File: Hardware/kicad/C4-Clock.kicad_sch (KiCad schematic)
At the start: 39 parts, among them J1 Keypad, J2 Battery, J3 LCD1602, J4 Boost Module, J5 ICSP, K1 FINDER-36.11-5V, Q1 S9014, Q2 S9014, Q3 S9014, SW1 SW_SPST, SW2 SW_SPST, U1 ATmega328P-P, U2 AMS1117-5.0, U3 PCF8574A, U4 DS1302+, Y1 16MHz, Y2 32.768kHz

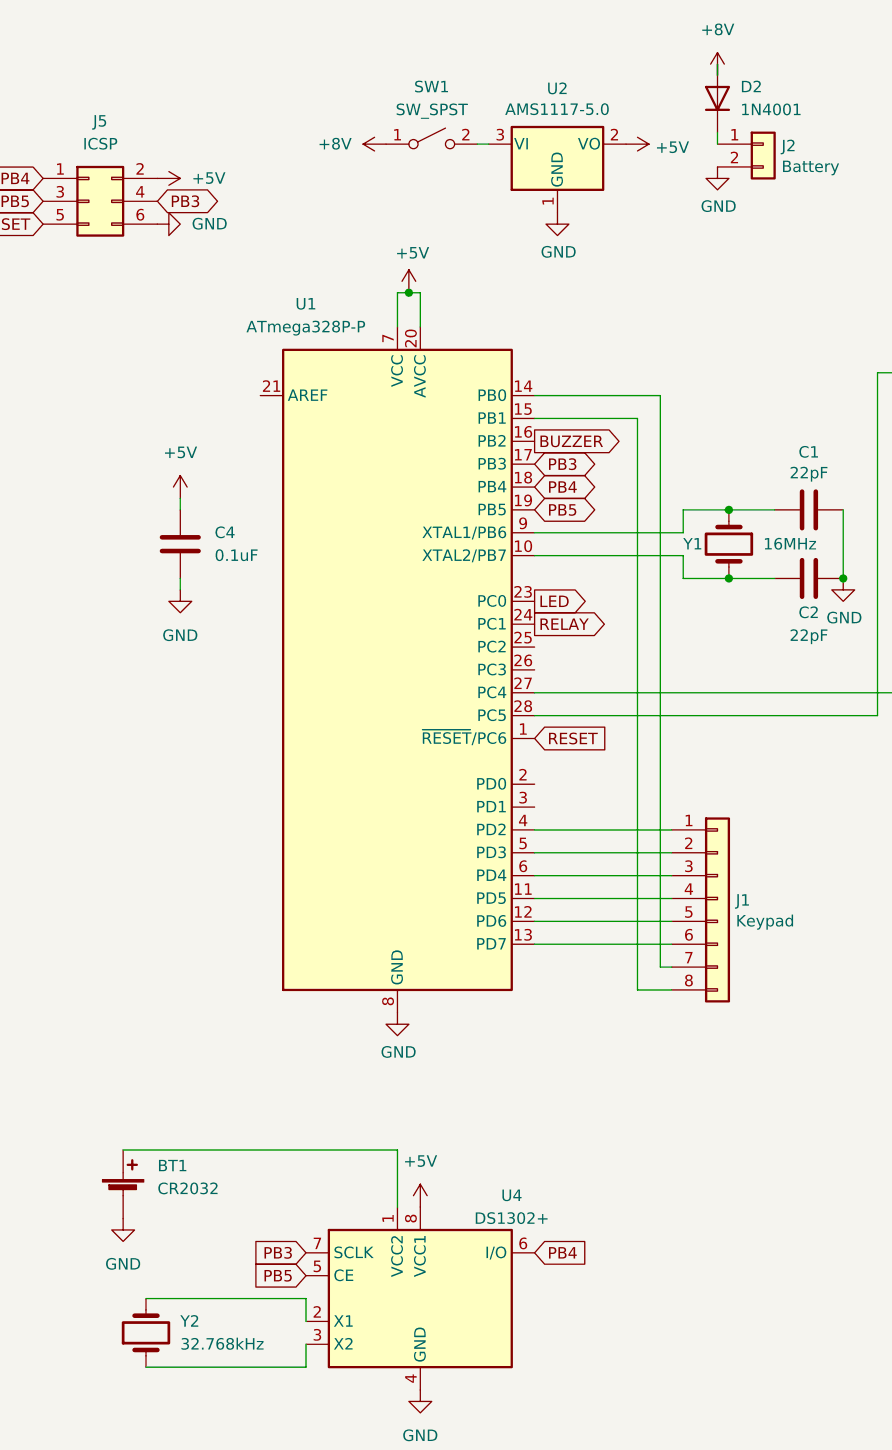
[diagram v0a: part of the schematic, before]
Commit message: hardware: Update PCB
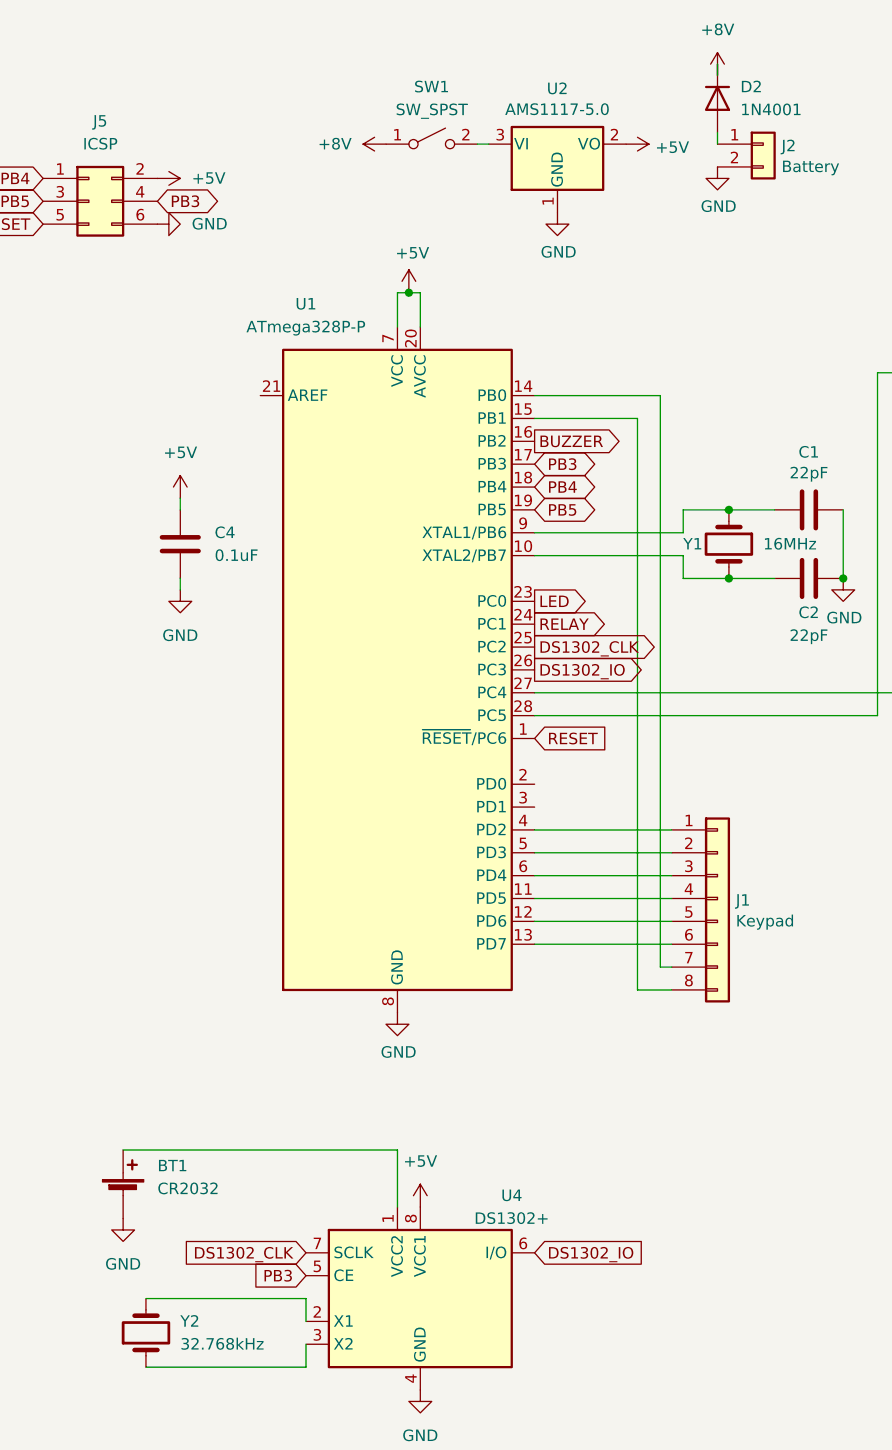
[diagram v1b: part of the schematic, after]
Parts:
- U4: footprint Package_DIP:DIP-8_W7.62mm -> Package_DIP:DIP-8_W7.62mm_Socket
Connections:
- net +8V: now also D2.1 (K); no longer D2.2 (A)
- net PB3: now also U4.5 (CE); no longer U4.7 (SCLK)
- net PB4: no longer U4.6 (I/O)
- net PB5: no longer U4.5 (CE)
- net at J2.1 (Pin_1): now also D2.2 (A); no longer D2.1 (K)
- net DS1302_CLK: now reaches U1.25 (PC2)
- net DS1302_CLK: now also U4.7 (SCLK)
- net DS1302_IO: now reaches U1.26 (PC3)
- net DS1302_IO: now also U4.6 (I/O)
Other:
- moved on the sheet: D2
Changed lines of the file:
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@@
     )
   )
-  (global_label "PB4" (shape input) (at 85.09 151.13 0) (fields_autoplaced)
+  (global_label "DS1302_IO" (shape input) (at 85.09 151.13 0) (fields_autoplaced)
     (effects (font (size 1.27 1.27)) (justify left))
-    (property "Intersheet References" "${INTERSHEET_REFS}" (id 0) (at 91.1637 151.0506 0)
+    (property "Intersheet References" "${INTERSHEET_REFS}" (id 0) (at 97.6347 151.0506 0)
       (effects (font (size 1.27 1.27)) (justify left) hide)
     )
@@
     )
   )
+  (global_label "DS1302_IO" (shape output) (at 85.09 86.36 0) (fields_autoplaced)
+    (effects (font (size 1.27 1.27)) (justify left))
+    (property "Intersheet References" "${INTERSHEET_REFS}" (id 0) (at 97.6347 86.2806 0)
+      (effects (font (size 1.27 1.27)) (justify left) hide)
+    )
+  )
   (global_label "BUZZER" (shape input) (at 139.7 113.03 180) (fields_autoplaced)
     (effects (font (size 1.27 1.27)) (justify right))
@@
     )
   )
-  (global_label "PB5" (shape input) (at 59.69 153.67 180) (fields_autoplaced)
+  (global_label "PB3" (shape input) (at 59.69 153.67 180) (fields_autoplaced)
     (effects (font (size 1.27 1.27)) (justify right))
     (property "Intersheet References" "${INTERSHEET_REFS}" (id 0) (at 53.6163 153.5906 0)
       (effects (font (size 1.27 1.27)) (justify right) hide)
+    )
+  )
+  (global_label "DS1302_CLK" (shape output) (at 85.09 83.82 0) (fields_autoplaced)
+    (effects (font (size 1.27 1.27)) (justify left))
+    (property "Intersheet References" "${INTERSHEET_REFS}" (id 0) (at 99.2675 83.7406 0)
+      (effects (font (size 1.27 1.27)) (justify left) hide)
     )
   )
@@
     )
   )
-  (global_label "PB3" (shape input) (at 59.69 151.13 180) (fields_autoplaced)
+  (global_label "DS1302_CLK" (shape input) (at 59.69 151.13 180) (fields_autoplaced)
     (effects (font (size 1.27 1.27)) (justify right))
-    (property "Intersheet References" "${INTERSHEET_REFS}" (id 0) (at 53.6163 151.0506 0)
+    (property "Intersheet References" "${INTERSHEET_REFS}" (id 0) (at 45.5125 151.0506 0)
       (effects (font (size 1.27 1.27)) (justify right) hide)
     )
@@
     (pin "1")
   )
-  (symbol (lib_id "Diode:1N4001") (at 105.41 22.86 90) (unit 1)
+  (symbol (lib_id "Diode:1N4001") (at 105.41 22.86 270) (unit 1)
     (in_bom yes) (on_board yes) (fields_autoplaced)
     (property "Reference" "D2" (id 0) (at 107.95 21.5899 90)
-      (effects (font (size 1.27 1.27)) (justify right))
+      (effects (font (size 1.27 1.27)) (justify left))
     )
     (property "Value" "1N4001" (id 1) (at 107.95 24.1299 90)
-      (effects (font (size 1.27 1.27)) (justify right))
-    )
-    (property "Footprint" "Diode_THT:D_DO-41_SOD81_P10.16mm_Horizontal" (id 2) (at 109.855 22.86 0)
+      (effects (font (size 1.27 1.27)) (justify left))
+    )
+    (property "Footprint" "Diode_THT:D_DO-41_SOD81_P10.16mm_Horizontal" (id 2) (at 100.965 22.86 0)
       (effects (font (size 1.27 1.27)) hide)
     )
@@
     (property "Reference" "U4" (id 0) (at 82.55 144.78 0))
     (property "Value" "DS1302+" (id 1) (at 82.55 147.32 0))
-    (property "Footprint" "Package_DIP:DIP-8_W7.62mm" (id 2) (at 72.39 168.91 0)
+    (property "Footprint" "Package_DIP:DIP-8_W7.62mm_Socket" (id 2) (at 72.39 168.91 0)
       (effects (font (size 1.27 1.27)) hide)
     )
@@
     )
     (path "/9c8b409b-0d1b-49e5-8fed-acd83e0e8b3e"
-      (reference "U4") (unit 1) (value "DS1302+") (footprint "Package_DIP:DIP-8_W7.62mm")
+      (reference "U4") (unit 1) (value "DS1302+") (footprint "Package_DIP:DIP-8_W7.62mm_Socket")
     )
     (path "/00000000-0000-0000-0000-0000621ca23f"
